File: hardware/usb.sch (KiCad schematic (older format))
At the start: 17 parts, among them J901 USB_OTG, U901 NX5P3090, U902 SMP1255PUTG, U903 USB3320, U904 OSC

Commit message: Fixed Schematic Symbols
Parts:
- C902, C903, C904, C905, C906, C907: symbol device:C_Small -> Device:C_Small
- J901: symbol conn:USB_OTG -> Connector:USB_OTG
- R901, R902, R903, R904, R905: symbol device:R -> Device:R
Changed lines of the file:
@@
 $Descr A4 11693 8268
 encoding utf-8
-Sheet 9 22
+Sheet 8 21
 Title ""
 Date ""
@@
 CLK
 $Comp
-L power1:GND #PWR096
+L power:GND #PWR096
 U 1 1 59921269
 P 7100 5100
@@
 NoConn ~ 6100 4700
 $Comp
-L device:R R905
+L Device:R R905
 U 1 1 59921EA9
 P 8250 4700
@@
 $EndComp
 $Comp
-L power1:GND #PWR097
+L power:GND #PWR097
 U 1 1 59921EDC
 P 8500 4800
@@
 	8500 4700 8500 4800
 $Comp
-L power1:GND #PWR098
+L power:GND #PWR098
 U 1 1 59921F43
 P 1200 4700
@@
 $EndComp
 $Comp
-L device:R R901
+L Device:R R901
 U 1 1 59922379
 P 1000 4550
@@
 $EndComp
 $Comp
-L power1:GND #PWR099
+L power:GND #PWR099
 U 1 1 599223A7
 P 1000 4700
@@
 $EndComp
 $Comp
-L device:R R904
+L Device:R R904
 U 1 1 599227D7
 P 5750 3600
@@
 	1200 4200 1200 4700
 $Comp
-L power1:GND #PWR0100
+L power:GND #PWR0100
 U 1 1 599229B3
 P 1850 4700
@@
 $EndComp
 $Comp
-L power1:+1V8 #PWR0101
+L power:+1V8 #PWR0101
 U 1 1 59922E8F
 P 6850 1600
@@
 	6850 1600 6850 1650
 $Comp
-L power1:+1V8 #PWR0102
+L power:+1V8 #PWR0102
 U 1 1 599243A9
 P 7350 1600
@@
 $EndComp
 $Comp
-L power1:GND #PWR0103
+L power:GND #PWR0103
 U 1 1 5992454D
 P 7350 2000
@@
 $EndComp
 $Comp
-L power1:GND #PWR0104
+L power:GND #PWR0104
 U 1 1 5992459D
 P 6850 2000
@@
 	6850 1650 7100 1650
 $Comp
-L power1:+3V3 #PWR0105
+L power:+3V3 #PWR0105
 U 1 1 59924C11
 P 6400 1600
@@
 $EndComp
 $Comp
-L power1:GND #PWR0106
+L power:GND #PWR0106
 U 1 1 59924C37
 P 6400 2000
@@
 Connection ~ 4700 4700
 $Comp
-L power1:GND #PWR0107
+L power:GND #PWR0107
 U 1 1 5A984E78
 P 4700 4800
@@
 $EndComp
 $Comp
-L power1:GND #PWR0108
+L power:GND #PWR0108
 U 1 1 5A985319
 P 3100 3400
@@
 	5350 3500 6100 3500
 $Comp
-L power1:GND #PWR0109
+L power:GND #PWR0109
 U 1 1 5A985418
 P 4700 2900
@@
 $EndComp
 $Comp
-L power1:+5V #PWR0110
+L power:+5V #PWR0110
 U 1 1 5A985450
 P 4700 2400
@@
 	4700 4600 4700 4700
 $Comp
-L device:R R902
+L Device:R R902
 U 1 1 5A985A8D
 P 4650 3200
@@
 $EndComp
 $Comp
-L power1:GND #PWR0111
+L power:GND #PWR0111
 U 1 1 5A985AE5
 P 4800 3200
@@
 ILIM current limit adjustment resistor:\nR=100k for I_ocp=581 mA typ.
 $Comp
-L device:R R903
+L Device:R R903
 U 1 1 5A986061
 P 5150 3100
@@
 Connection ~ 5150 3300
 $Comp
-L power1:+1V8 #PWR0112
+L power:+1V8 #PWR0112
 U 1 1 5A9861C7
 P 5150 2950
@@
 	10100 4150 10000 4150
 $Comp
-L power1:GND #PWR0113
+L power:GND #PWR0113
 U 1 1 5A98862B
 P 8900 4250
@@
 Connection ~ 10050 3800
 $Comp
-L power1:+1V8 #PWR0114
+L power:+1V8 #PWR0114
 U 1 1 5A9888CB
 P 10050 3700
@@
 $EndComp
 $Comp
-L power1:GND #PWR0115
+L power:GND #PWR0115
 U 1 1 5A988966
 P 10350 4250
@@
 $EndComp
 $Comp
-L power1:GND #PWR0116
+L power:GND #PWR0116
 U 1 1 5A988E5D
 P 6000 3300
@@
 	7800 1600 7800 1650
 $Comp
-L power1:GND #PWR0117
+L power:GND #PWR0117
 U 1 1 5A989692
 P 7800 2000
@@
 Oscillator: DSC6003CI2A-012.0000\n(12 MHz)
 $Comp
-L conn:USB_OTG J901
+L Connector:USB_OTG J901
 U 1 1 5ACE0B3C
 P 1200 3800
@@
 	1100 4300 1100 4200
 $Comp
-L power1:+3V3 #PWR0118
+L power:+3V3 #PWR0118
 U 1 1 5B1F6406
 P 7800 1600
@@
 	2800 4500 3000 4500
 $Comp
-L device:C_Small C904
+L Device:C_Small C904
 U 1 1 5B2225E7
 P 6850 1850
@@
 $EndComp
 $Comp
-L device:C_Small C905
+L Device:C_Small C905
 U 1 1 5B224CCE
 P 7350 1850
@@
 $EndComp
 $Comp
-L device:C_Small C906
+L Device:C_Small C906
 U 1 1 5B224D20
 P 7800 1850
@@
 $EndComp
 $Comp
-L device:C_Small C907
+L Device:C_Small C907
 U 1 1 5B224D9D
 P 10350 4100
@@
 $EndComp
 $Comp
-L device:C_Small C902
+L Device:C_Small C902
 U 1 1 5B224E9D
 P 4700 2750
@@
 	10350 3800 10350 4000
 $Comp
-L device:C_Small C903
+L Device:C_Small C903
 U 1 1 5B23D5EF
 P 6400 1850

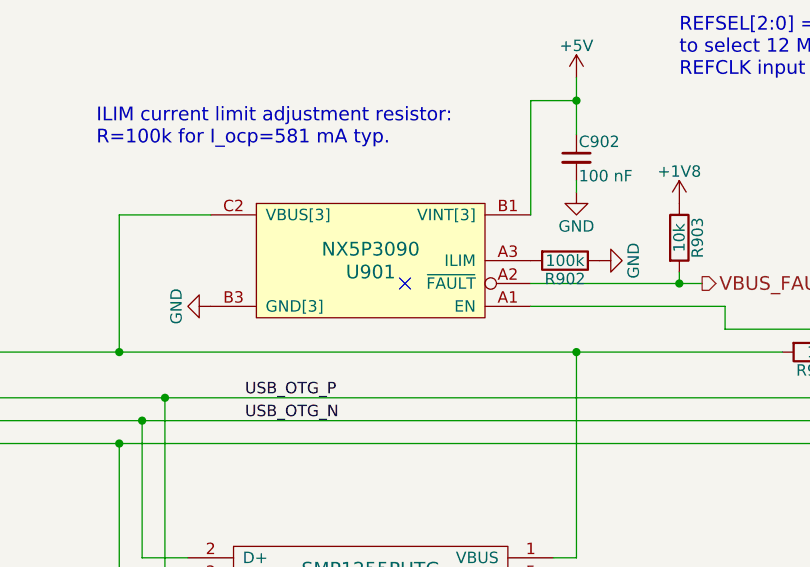
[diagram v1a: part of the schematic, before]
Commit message: WIP: TLK Powerdistribution
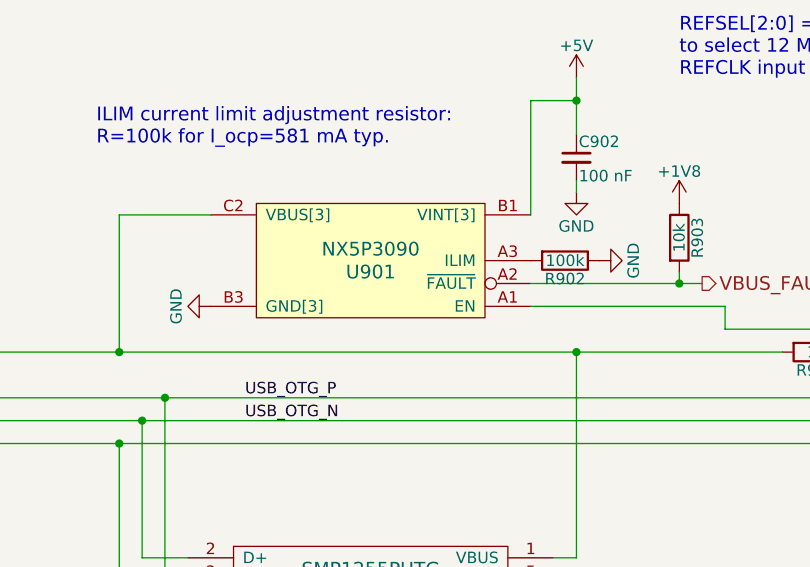
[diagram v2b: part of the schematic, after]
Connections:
- no-connect marks 4 -> 3
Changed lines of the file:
@@
 EESchema Schematic File Version 4
-LIBS:zynq_board-cache
 EELAYER 26 0
 EELAYER END
@@
 	1    0    0    -1
 $EndComp
-NoConn ~ 3950 3300
 Text Notes 700  3000 0    60   ~ 0
 TODO: correct MicroUSB Footprint
